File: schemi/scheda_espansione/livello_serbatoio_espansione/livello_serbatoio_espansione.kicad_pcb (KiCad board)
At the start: 2 copper layers, 70 x 50 mm, 264 parts, among them J1 exp1, J2 exp_spi, J3 exp2

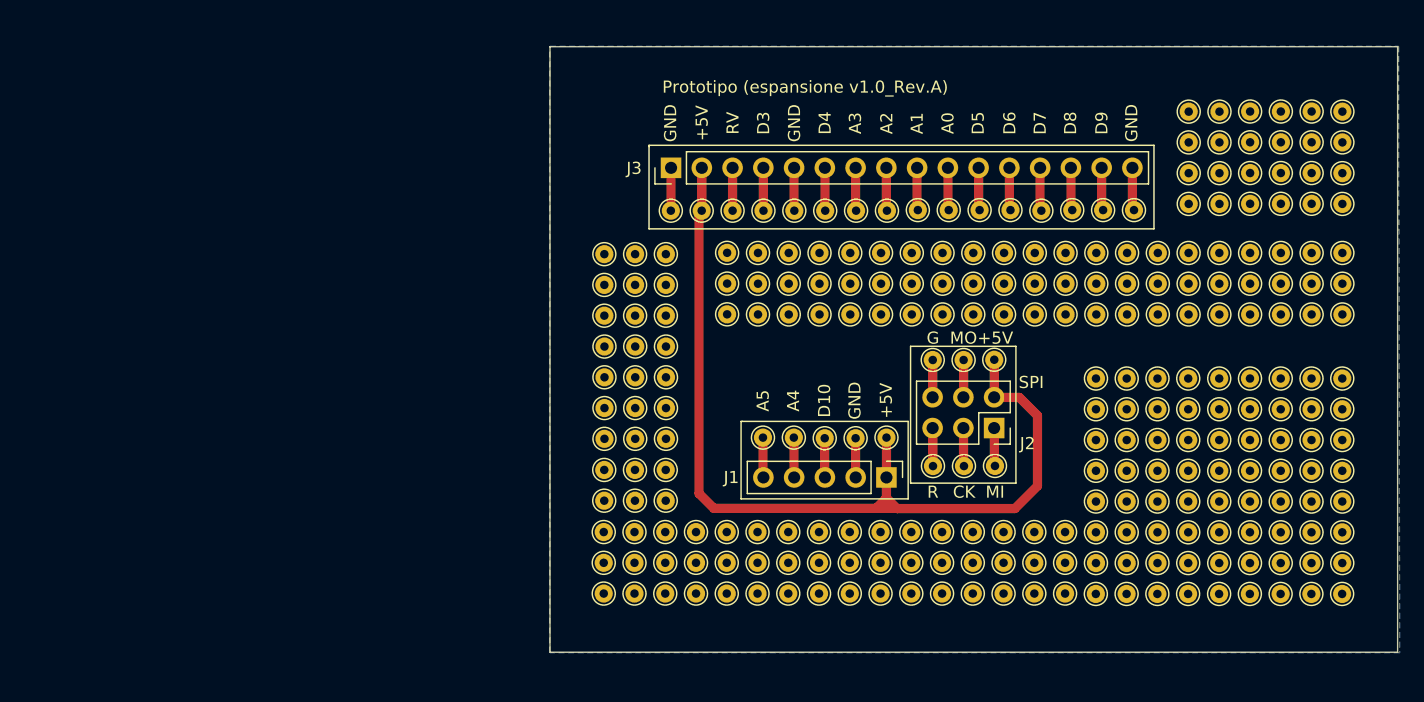
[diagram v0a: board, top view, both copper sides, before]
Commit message: modifiche scheda definitiva (rev. C)
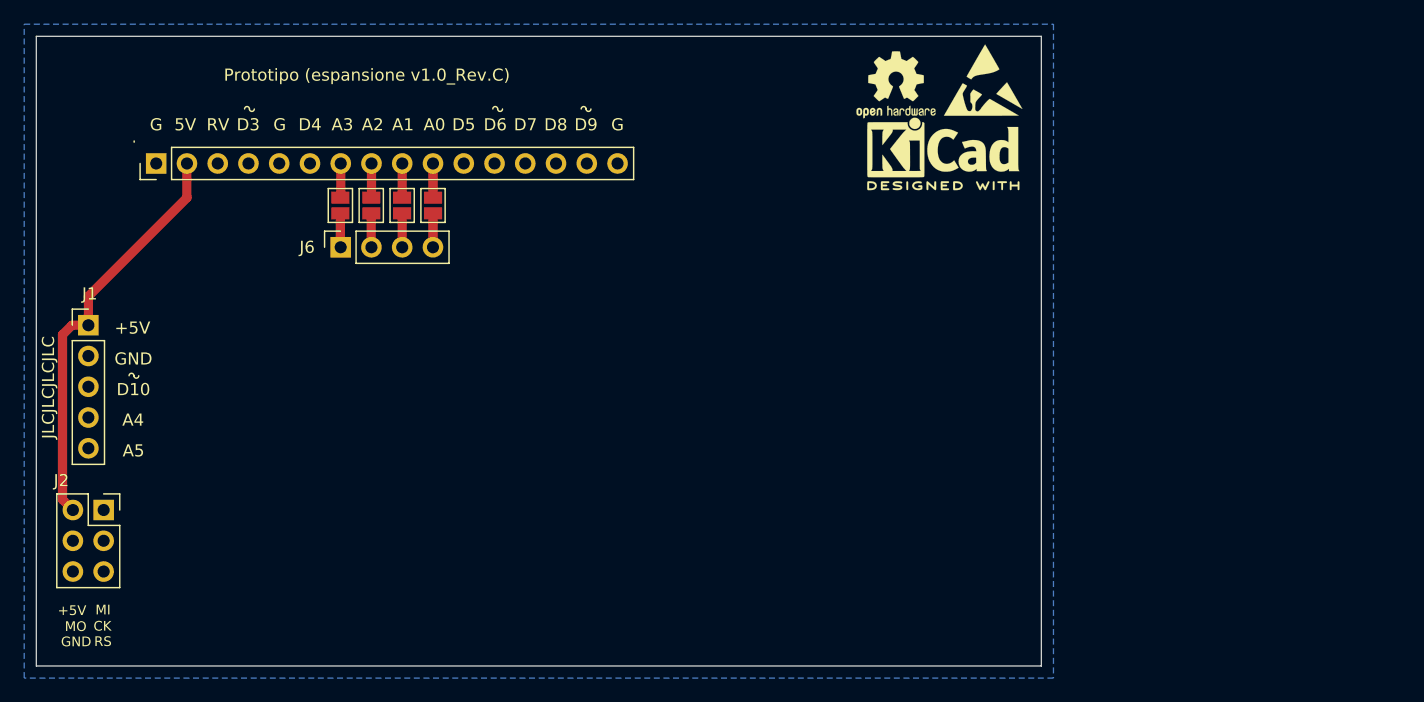
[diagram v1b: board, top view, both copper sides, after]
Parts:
- removed the REF** at (123.0, 62.9)
- removed the REF** at (156.0, 91.0)
- removed the REF** at (112.9, 78.2)
- removed the REF** at (171.3, 58.8)
- removed the REF** at (168.8, 58.8)
- removed the REF** at (166.2, 58.8)
- removed the REF** at (163.7, 58.8)
- removed the REF** at (161.2, 58.8)
- removed the REF** at (173.9, 58.8)
- removed the REF** at (173.8, 80.9)
- removed the REF** at (171.3, 80.9)
- removed the REF** at (168.8, 80.9)
- removed the REF** at (163.7, 91.0)
- removed the REF** at (166.2, 80.9)
- removed the REF** at (163.7, 80.9)
- removed the REF** at (161.1, 78.3)
- removed the REF** at (158.6, 78.3)
- removed the REF** at (156.1, 78.3)
- removed the REF** at (153.5, 78.3)
- removed the REF** at (118.0, 75.7)
- removed the REF** at (115.5, 75.7)
- removed the REF** at (112.9, 75.7)
- removed the REF** at (171.3, 56.3)
- removed the REF** at (171.3, 91.0)
- removed the REF** at (168.8, 56.3)
- removed the REF** at (166.2, 56.3)
- removed the REF** at (163.7, 56.3)
- removed the REF** at (161.2, 56.3)
- removed the REF** at (173.9, 56.3)
- removed the REF** at (173.8, 78.3)
- removed the REF** at (171.3, 78.3)
- removed the REF** at (168.8, 78.3)
- removed the REF** at (166.2, 78.3)
- removed the REF** at (163.7, 78.3)
- removed the REF** at (166.2, 91.0)
- removed the REF** at (161.1, 75.8)
- removed the REF** at (158.6, 75.8)
- removed the REF** at (156.1, 75.8)
- removed the REF** at (153.5, 75.8)
- removed the REF** at (118.0, 73.2)
- removed the REF** at (115.5, 73.2)
- removed the REF** at (112.9, 73.2)
- removed the REF** at (171.3, 53.8)
- removed the REF** at (168.8, 53.8)
- removed the REF** at (166.2, 53.8)
- removed the REF** at (153.5, 91.0)
- removed the REF** at (163.7, 53.8)
- removed the REF** at (161.2, 53.8)
- removed the REF** at (173.9, 53.8)
- removed the REF** at (173.8, 75.8)
- removed the REF** at (171.3, 75.8)
- removed the REF** at (168.8, 75.8)
- removed the REF** at (166.2, 75.8)
- removed the REF** at (163.7, 75.8)
- removed the REF** at (161.1, 73.3)
- removed the REF** at (158.6, 73.3)
- removed the REF** at (158.6, 91.0)
- removed the REF** at (156.1, 73.3)
- removed the REF** at (153.5, 73.3)
- removed the REF** at (118.0, 70.6)
- removed the REF** at (115.5, 70.6)
- removed the REF** at (112.9, 70.6)
- removed the REF** at (171.3, 51.2)
- removed the REF** at (168.8, 51.2)
- removed the REF** at (166.2, 51.2)
- removed the REF** at (163.7, 51.2)
- removed the REF** at (161.2, 51.2)
- removed the REF** at (161.1, 91.0)
- removed the REF** at (173.9, 51.2)
- removed the REF** at (173.8, 73.3)
- removed the REF** at (171.3, 73.3)
- removed the REF** at (168.8, 73.3)
- removed the REF** at (166.2, 73.3)
- removed the REF** at (163.7, 73.3)
- removed the REF** at (173.9, 68.0)
- removed the REF** at (171.3, 68.0)
- removed the REF** at (168.8, 68.0)
- removed the REF** at (166.2, 68.0)
- removed the REF** at (168.8, 91.0)
- removed the REF** at (163.7, 68.0)
- removed the REF** at (161.2, 68.0)
- removed the REF** at (158.6, 68.0)
- removed the REF** at (156.1, 68.0)
- removed the REF** at (153.5, 68.0)
- removed the REF** at (151.0, 68.0)
- removed the REF** at (148.5, 68.0)
- removed the REF** at (145.9, 68.0)
- removed the REF** at (143.4, 68.0)
- removed the REF** at (140.8, 68.0)
- removed the REF** at (173.8, 91.0)
- removed the REF** at (138.3, 68.0)
- removed the REF** at (135.8, 68.0)
- removed the REF** at (133.2, 68.0)
- removed the REF** at (130.7, 68.0)
- removed the REF** at (128.1, 68.0)
- removed the REF** at (125.6, 68.0)
- removed the REF** at (118.0, 68.1)
- removed the REF** at (115.5, 68.1)
- removed the REF** at (112.9, 68.1)
- removed the REF** at (173.9, 65.4)
- removed the REF** at (161.1, 88.5)
- removed the REF** at (171.3, 65.4)
- removed the REF** at (168.8, 65.4)
- removed the REF** at (166.2, 65.4)
- removed the REF** at (163.7, 65.4)
- removed the REF** at (161.2, 65.4)
- removed the REF** at (158.6, 65.4)
- removed the REF** at (156.1, 65.4)
- removed the REF** at (153.5, 65.4)
- removed the REF** at (151.0, 65.4)
- removed the REF** at (148.5, 65.4)
- removed the REF** at (123.0, 65.4)
- removed the REF** at (158.6, 88.5)
- removed the REF** at (145.9, 65.4)
- removed the REF** at (143.4, 65.4)
- removed the REF** at (140.8, 65.4)
- removed the REF** at (138.3, 65.4)
- removed the REF** at (135.8, 65.4)
- removed the REF** at (133.2, 65.4)
- removed the REF** at (130.7, 65.4)
- removed the REF** at (128.1, 65.4)
- removed the REF** at (125.6, 65.4)
- removed the REF** at (118.0, 65.5)
- removed the REF** at (156.1, 88.5)
- removed the REF** at (115.5, 65.5)
- removed the REF** at (112.9, 65.5)
- removed the REF** at (173.9, 62.9)
- removed the REF** at (171.3, 62.9)
- removed the REF** at (168.8, 62.9)
- removed the REF** at (166.2, 62.9)
- removed the REF** at (163.7, 62.9)
- removed the REF** at (161.2, 62.9)
- removed the REF** at (158.6, 62.9)
- removed the REF** at (156.1, 62.9)
- removed the REF** at (153.5, 88.5)
- removed the REF** at (153.5, 62.9)
- removed the REF** at (151.0, 62.9)
- removed the REF** at (148.5, 62.9)
- removed the REF** at (145.9, 62.9)
- removed the REF** at (143.4, 62.9)
- removed the REF** at (140.8, 62.9)
- removed the REF** at (138.3, 62.9)
- removed the REF** at (135.8, 62.9)
- removed the REF** at (133.2, 62.9)
- removed the REF** at (130.7, 62.9)
- removed the REF** at (151.0, 91.0)
- removed the REF** at (128.1, 62.9)
- removed the REF** at (125.6, 62.9)
- removed the REF** at (118.0, 63.0)
- removed the REF** at (115.5, 63.0)
- removed the REF** at (112.9, 63.0)
- removed the REF** at (148.4, 91.0)
- removed the REF** at (145.9, 91.0)
- removed the REF** at (143.3, 91.0)
- removed the REF** at (140.8, 91.0)
- removed the REF** at (138.3, 91.0)
- removed the REF** at (135.7, 91.0)
- removed the REF** at (123.0, 68.0)
- removed the REF** at (133.2, 91.0)
- removed the REF** at (130.6, 91.0)
- removed the REF** at (128.1, 91.0)
- removed the REF** at (125.6, 91.0)
- removed the REF** at (123.0, 91.0)
- removed the REF** at (120.5, 91.0)
- removed the REF** at (117.9, 91.0)
- removed the REF** at (115.4, 91.0)
- removed the REF** at (112.9, 91.0)
- removed the REF** at (173.8, 88.5)
- removed the REF** at (115.4, 83.3)
- removed the REF** at (171.3, 88.5)
- removed the REF** at (168.8, 88.5)
- removed the REF** at (166.2, 88.5)
- removed the REF** at (163.7, 88.5)
- removed the REF** at (161.1, 86.0)
- removed the REF** at (158.6, 86.0)
- removed the REF** at (156.1, 86.0)
- removed the REF** at (153.5, 86.0)
- removed the REF** at (151.0, 88.5)
- removed the REF** at (148.4, 88.5)
- removed the REF** at (112.9, 80.8)
- removed the REF** at (145.9, 88.5)
- removed the REF** at (143.3, 88.5)
- removed the REF** at (140.8, 88.5)
- removed the REF** at (138.3, 88.5)
- removed the REF** at (135.7, 88.5)
- removed the REF** at (133.2, 88.5)
- removed the REF** at (130.6, 88.5)
- removed the REF** at (128.1, 88.5)
- removed the REF** at (125.6, 88.5)
- removed the REF** at (123.0, 88.5)
- removed the REF** at (118.0, 80.8)
- removed the REF** at (120.5, 88.5)
- removed the REF** at (117.9, 88.5)
- removed the REF** at (115.4, 88.5)
- removed the REF** at (112.9, 88.5)
- removed the REF** at (173.8, 86.0)
- removed the REF** at (171.3, 86.0)
- removed the REF** at (168.8, 86.0)
- removed the REF** at (166.2, 86.0)
- removed the REF** at (163.7, 86.0)
- removed the REF** at (161.1, 83.4)
- removed the REF** at (115.4, 80.8)
- removed the REF** at (158.6, 83.4)
- removed the REF** at (156.1, 83.4)
- removed the REF** at (153.5, 83.4)
- removed the REF** at (151.0, 85.9)
- removed the REF** at (148.4, 85.9)
- removed the REF** at (145.9, 85.9)
- removed the REF** at (143.3, 85.9)
- removed the REF** at (140.8, 85.9)
- removed the REF** at (138.3, 85.9)
- removed the REF** at (135.7, 85.9)
- removed the REF** at (112.9, 83.3)
- removed the REF** at (133.2, 85.9)
- removed the REF** at (130.6, 85.9)
- removed the REF** at (128.1, 85.9)
- removed the REF** at (125.6, 85.9)
- removed the REF** at (123.0, 85.9)
- removed the REF** at (120.5, 85.9)
- removed the REF** at (117.9, 85.9)
- removed the REF** at (115.4, 85.9)
- removed the REF** at (112.9, 85.9)
- removed the REF** at (173.8, 83.4)
- removed the REF** at (118.0, 83.3)
- removed the REF** at (171.3, 83.4)
- removed the REF** at (168.8, 83.4)
- removed the REF** at (166.2, 83.4)
- removed the REF** at (163.7, 83.4)
- removed the REF** at (161.1, 80.9)
- removed the REF** at (158.6, 80.9)
- removed the REF** at (156.1, 80.9)
- removed the REF** at (153.5, 80.9)
- removed the REF** at (118.0, 78.2)
- removed the REF** at (115.5, 78.2)
- removed TP1, TP12, TP23, TP27, TP5: GND, TestPoint:TestPoint_THTPad_D1.5mm_Drill0.7mm
- removed TP10: SPI_SCK, TestPoint:TestPoint_THTPad_D1.5mm_Drill0.7mm
- removed TP11: SPI_MISO, TestPoint:TestPoint_THTPad_D1.5mm_Drill0.7mm
- removed TP13: D9, TestPoint:TestPoint_THTPad_D1.5mm_Drill0.7mm
- removed TP14: D8, TestPoint:TestPoint_THTPad_D1.5mm_Drill0.7mm
- removed TP15: D7, TestPoint:TestPoint_THTPad_D1.5mm_Drill0.7mm
- removed TP16: D6, TestPoint:TestPoint_THTPad_D1.5mm_Drill0.7mm
- removed TP17: D5, TestPoint:TestPoint_THTPad_D1.5mm_Drill0.7mm
- removed TP18: A0, TestPoint:TestPoint_THTPad_D1.5mm_Drill0.7mm
- removed TP19: A1, TestPoint:TestPoint_THTPad_D1.5mm_Drill0.7mm
- removed TP2: SPI_MOSI, TestPoint:TestPoint_THTPad_D1.5mm_Drill0.7mm
- removed TP20: A2, TestPoint:TestPoint_THTPad_D1.5mm_Drill0.7mm
- removed TP21: A3, TestPoint:TestPoint_THTPad_D1.5mm_Drill0.7mm
- removed TP22: D4, TestPoint:TestPoint_THTPad_D1.5mm_Drill0.7mm
- removed TP24: D3, TestPoint:TestPoint_THTPad_D1.5mm_Drill0.7mm
- removed TP25: RV, TestPoint:TestPoint_THTPad_D1.5mm_Drill0.7mm
- removed TP26, TP3: VDD, TestPoint:TestPoint_THTPad_D1.5mm_Drill0.7mm
- removed TP4: +5V, TestPoint:TestPoint_THTPad_D1.5mm_Drill0.7mm
- removed TP6: D10, TestPoint:TestPoint_THTPad_D1.5mm_Drill0.7mm
- removed TP7: A4, TestPoint:TestPoint_THTPad_D1.5mm_Drill0.7mm
- removed TP8: A5, TestPoint:TestPoint_THTPad_D1.5mm_Drill0.7mm
- removed TP9: RST, TestPoint:TestPoint_THTPad_D1.5mm_Drill0.7mm
- added J6: Exp_Analog_2, Connector_PinSocket_2.54mm:PinSocket_1x04_P2.54mm_Vertical, F.Cu at (91.1, 62.4)
- added JP1: A0_J, Jumper:SolderJumper-2_P1.3mm_Open_Pad1.0x1.5mm, F.Cu at (98.8, 59.0)
- added JP2: A1_J, Jumper:SolderJumper-2_P1.3mm_Open_Pad1.0x1.5mm, F.Cu at (96.2, 59.0)
- added JP3: A2_J, Jumper:SolderJumper-2_P1.3mm_Open_Pad1.0x1.5mm, F.Cu at (93.7, 59.0)
- added JP4: A3_J, Jumper:SolderJumper-2_P1.3mm_Open_Pad1.0x1.5mm, F.Cu at (91.1, 59.0)
- added REF**: OSHW-Logo2_7.3x6mm_SilkScreen, Symbol:OSHW-Logo2_7.3x6mm_SilkScreen, F.Cu at (137.0, 49.0)
- added REF**: KiCad-Logo2_5mm_SilkScreen, Symbol:KiCad-Logo2_5mm_SilkScreen, F.Cu at (140.9, 54.7)
- added REF**: ESD-Logo_6.6x6mm_SilkScreen, Symbol:ESD-Logo_6.6x6mm_SilkScreen, F.Cu at (144.2, 48.6)
- moved J2 73.9 mm to (71.6, 84.1), turned to 0 degrees
- moved J1 67.1 mm to (70.3, 68.9), turned to 0 degrees
- moved J3 42.5 mm to (75.9, 55.5)
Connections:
- J3 pad 10: A0 -> Net-(J3-Pin_10)
- J3 pad 7: A3 -> Net-(J3-Pin_7)
- J3 pad 8: A2 -> Net-(J3-Pin_8)
- J3 pad 9: A1 -> Net-(J3-Pin_9)
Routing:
- net VDD: track 76.8 -> 34.6 mm
- net GND: track 17.0 -> 0.01 mm
- net D7: track 3.58 -> 0.00 mm
- net D4: track 3.55 -> 0.00 mm
- net D3: track 3.54 -> 0.00 mm
- net RV: track 3.54 -> 0.00 mm
- net D9: track 3.54 -> 0.00 mm
- net D8: track 3.54 -> 0.00 mm
- net D6: track 3.53 -> 0.00 mm
- net D5: track 3.52 -> 0.00 mm
- net A4: track 3.30 -> 0.04 mm
- net A5: track 3.30 -> 0.05 mm
- net D10: track 3.25 -> 0.02 mm
- net SCK: track 3.14 -> 0.00 mm
- net MISO: track 3.14 -> 0.00 mm
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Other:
- board size 70 x 50 mm -> 83 x 52 mm
- net class Default removed
- board text added: "5V"
- board text added: "JLCJLCJLCJLC"
- board text added: "Prototipo (espansione v1.0_Rev.C)"
- board text added: "RS"
- board text removed: "Prototipo (espansione v1.0_Rev.A)"
- board text removed: "R"
- board text removed: "SPI"
